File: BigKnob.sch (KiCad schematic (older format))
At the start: 10 parts, among them J1 NSJ12HF-1, J2 NSJ12HF-1, J3 NSJ12HF-1, J4 STEREO-JACK-SWITCHED-5-Pin, J5 STEREO-JACK-SWITCHED-5-Pin

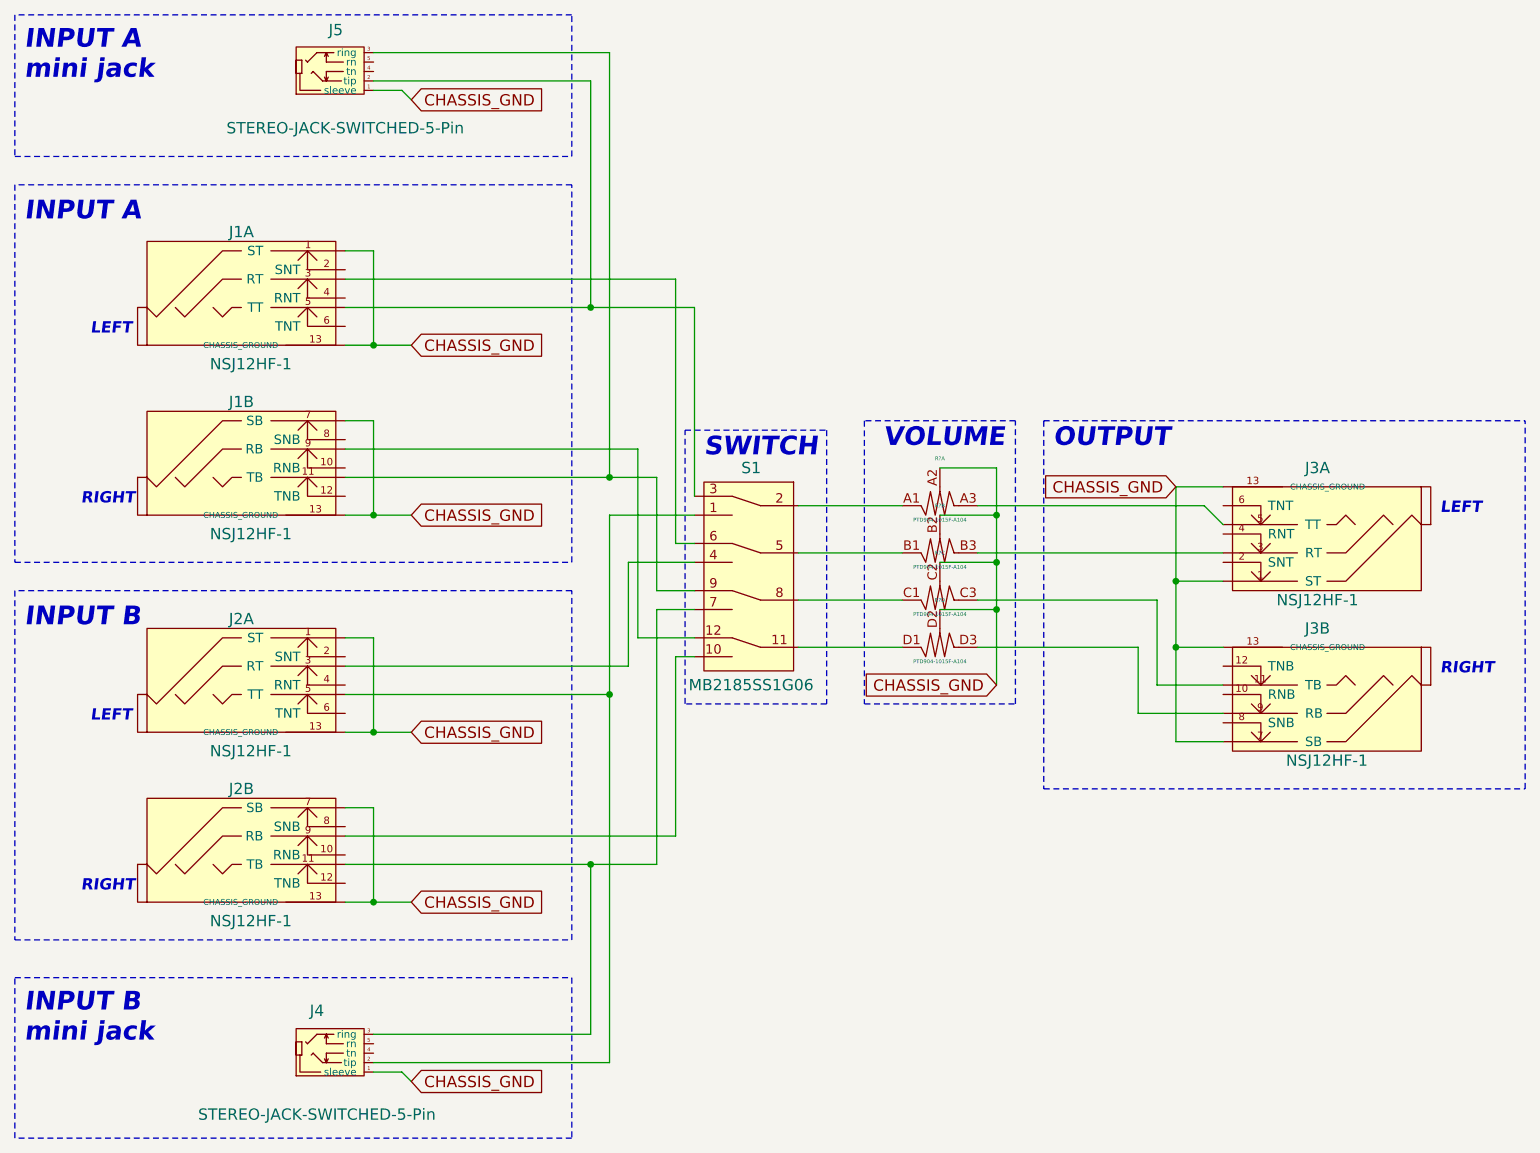
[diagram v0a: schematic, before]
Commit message: :punch: fixed schema
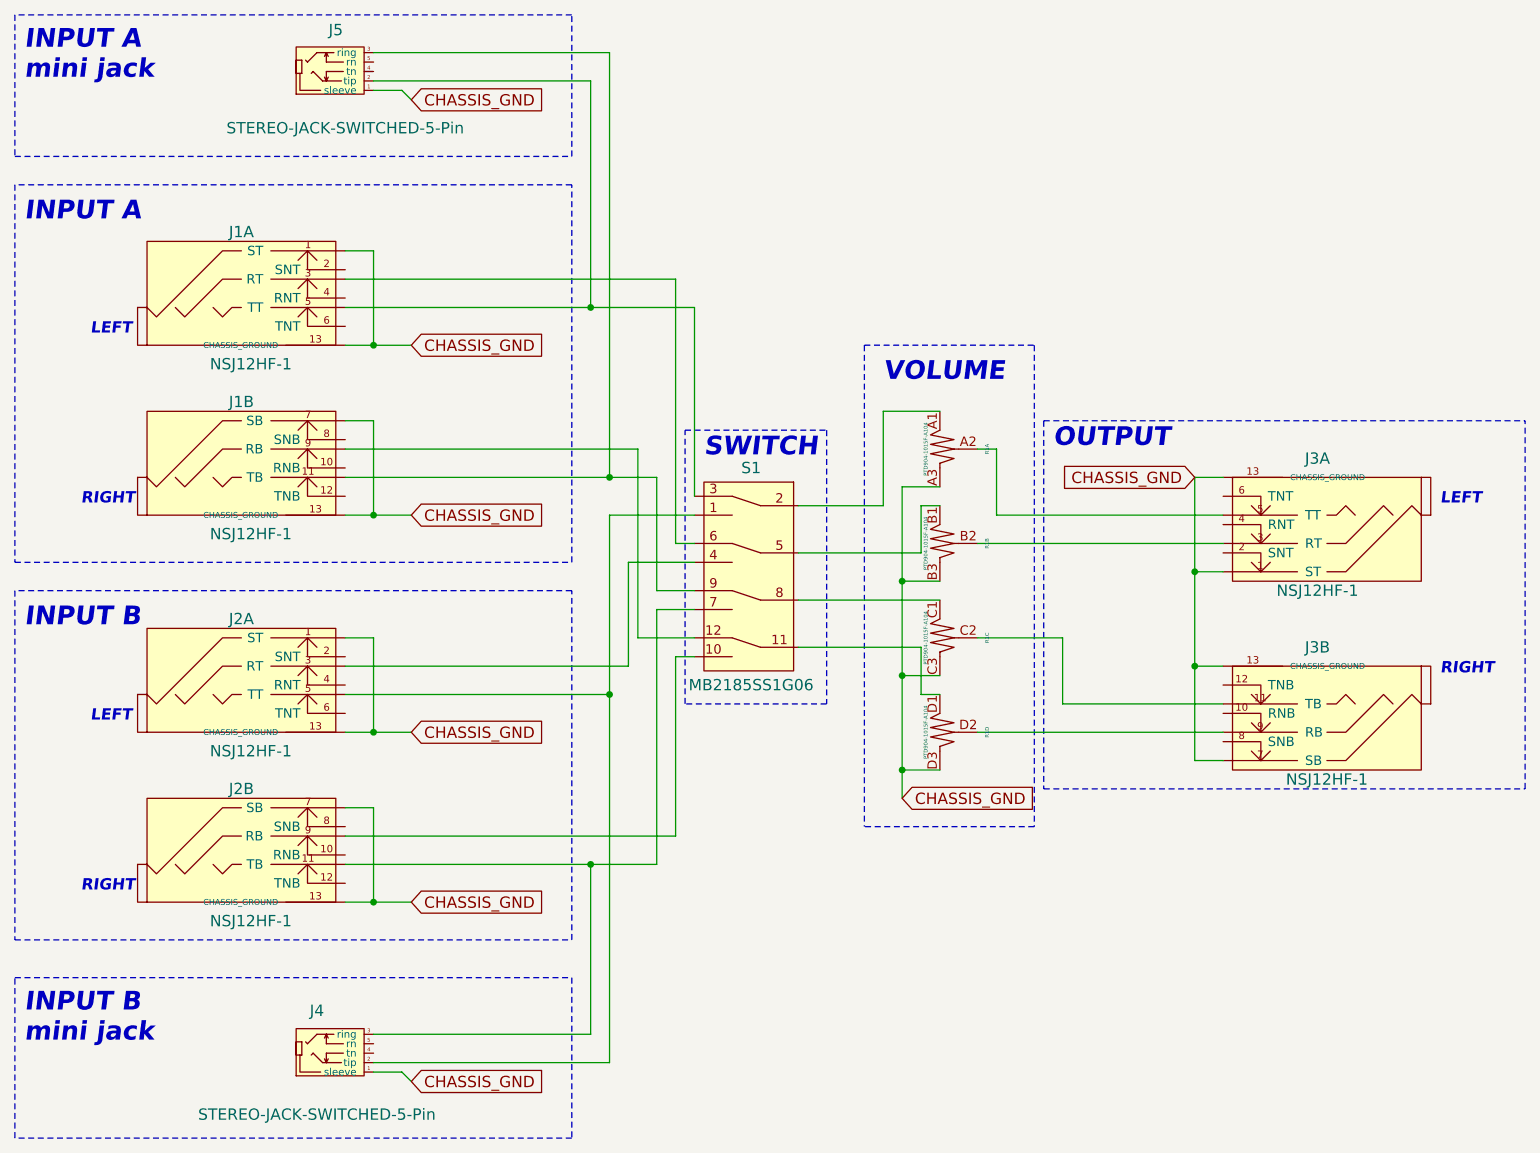
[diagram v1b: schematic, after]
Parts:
- R1: renamed from R?; footprint (none) -> stahllabs:PTD904-1015F-A104
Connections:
- net CHASSIS_GND: now also R1.A3, R1.B3, R1.C3, R1.D3; no longer R1.A2, R1.B2, R1.C2, R1.D2
- net at J3.3 (RT): now also R1.B2; no longer R1.B3
- net at J3.5 (TT): now also R1.A2; no longer R1.A3
- net at J3.11 (TB): now also R1.C2; no longer R1.C3
- net at J3.9 (RB): now also R1.D2; no longer R1.D3
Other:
- moved on the sheet: J3A, J3B, R1A, R1B, R1C, R1D
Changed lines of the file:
@@
 $EndComp
 Wire Wire Line
-	3150 2700 3300 2700
-Wire Wire Line
-	3300 2700 3500 2700
-Wire Wire Line
-	3150 3600 3300 3600
-Wire Wire Line
-	3300 3600 3500 3600
-Wire Wire Line
-	3150 4750 3300 4750
-Wire Wire Line
-	3300 4750 3500 4750
+	3150 2700 3500 2700
+Wire Wire Line
+	3150 3600 3500 3600
+Wire Wire Line
+	3150 4750 3500 4750
 Text GLabel 3500 2700 2    60   Input ~ 0
 CHASSIS_GND
@@
 CHASSIS_GND
 Wire Wire Line
-	3150 5650 3300 5650
-Wire Wire Line
-	3300 5650 3500 5650
+	3150 5650 3500 5650
 Text GLabel 3500 5650 2    60   Input ~ 0
 CHASSIS_GND
@@
 L NSJ12HF-1 J3
 U 1 1 58E15C9F
-P 8350 3750
-F 0 "J3" H 8400 3350 60  0000 C CNN
-F 1 "NSJ12HF-1" H 8400 4050 60  0000 C CNN
-F 2 "stahllabs:NSJ12HF-1" H 8700 3900 60  0001 C CNN
-F 3 "http://www.neutrik.com/en/audio/plugs-and-jacks/stacking-jacks/nsj12hf-1" H 8400 3250 21  0001 C BIN
-	1    8350 3750
+P 8350 3700
+F 0 "J3" H 8400 3300 60  0000 C CNN
+F 1 "NSJ12HF-1" H 8400 4000 60  0000 C CNN
+F 2 "stahllabs:NSJ12HF-1" H 8700 3850 60  0001 C CNN
+F 3 "http://www.neutrik.com/en/audio/plugs-and-jacks/stacking-jacks/nsj12hf-1" H 8400 3200 21  0001 C BIN
+	1    8350 3700
 	-1   0    0    1
 $EndComp
@@
 L NSJ12HF-1 J3
 U 2 1 58E15D3A
-P 8350 4600
-F 0 "J3" H 8400 4200 60  0000 C CNN
-F 1 "NSJ12HF-1" H 8350 4900 60  0000 C CNN
-F 2 "stahllabs:NSJ12HF-1" H 8700 4750 60  0001 C CNN
-F 3 "http://www.neutrik.com/en/audio/plugs-and-jacks/stacking-jacks/nsj12hf-1" H 8400 4100 21  0001 C BIN
-	2    8350 4600
+P 8350 4700
+F 0 "J3" H 8400 4300 60  0000 C CNN
+F 1 "NSJ12HF-1" H 8350 5000 60  0000 C CNN
+F 2 "stahllabs:NSJ12HF-1" H 8700 4850 60  0001 C CNN
+F 3 "http://www.neutrik.com/en/audio/plugs-and-jacks/stacking-jacks/nsj12hf-1" H 8400 4200 21  0001 C BIN
+	2    8350 4700
 	-1   0    0    1
 $EndComp
 Wire Wire Line
-	7450 4050 7450 4500
-Wire Wire Line
-	7450 4500 7800 4500
-Wire Wire Line
-	7350 4300 7350 4650
-Wire Wire Line
-	7350 4650 7800 4650
+	6950 4250 6950 4600
+Wire Wire Line
+	6950 4600 7800 4600
+Wire Wire Line
+	6500 4750 7800 4750
 Wire Wire Line
 	3150 4550 4550 4550
 Wire Wire Line
-	4550 3600 4550 4550
-Wire Wire Line
-	4550 4550 4550 6500
-Wire Wire Line
-	6500 3550 7700 3550
-Wire Wire Line
-	7700 3550 7800 3650
-Text Notes 8950 3600 0    60   Italic 12
+	4550 3600 4550 6500
+Text Notes 8950 3550 0    60   Italic 12
 LEFT
 Text Notes 1800 2650 0    60   Italic 12
@@
 RIGHT
 Wire Wire Line
-	6500 3800 7800 3800
-Wire Wire Line
-	7550 4300 7800 4300
-Wire Wire Line
-	7550 3450 7550 3950
-Wire Wire Line
-	7550 3950 7550 4300
-Wire Wire Line
-	7550 4300 7550 4800
-Wire Wire Line
-	7800 3950 7550 3950
-Connection ~ 7550 3950
-Wire Wire Line
-	7550 4800 7800 4800
-Connection ~ 7550 4300
-Wire Wire Line
-	6500 4050 7450 4050
-Wire Wire Line
-	6500 4300 7350 4300
+	7650 4400 7800 4400
+Wire Wire Line
+	7650 3400 7650 4900
+Wire Wire Line
+	7800 3900 7650 3900
+Connection ~ 7650 3900
+Wire Wire Line
+	7650 4900 7800 4900
+Connection ~ 7650 4400
 Text Notes 8950 4450 0    60   Italic 12
 RIGHT
 Wire Wire Line
-	3150 2500 4450 2500
-Wire Wire Line
-	4450 2500 5000 2500
+	3150 2500 5000 2500
 Wire Wire Line
 	5000 2500 5000 3500
@@
 Connection ~ 3300 3600
 Wire Wire Line
-	7550 3450 7800 3450
-Text GLabel 7550 3450 0    60   Input ~ 0
-CHASSIS_GND
-Wire Wire Line
-	3150 3400 4550 3400
-Wire Wire Line
-	4550 3400 4800 3400
+	7650 3400 7800 3400
+Text GLabel 7650 3400 0    60   Input ~ 0
+CHASSIS_GND
+Wire Wire Line
+	3150 3400 4800 3400
 Wire Wire Line
 	4800 3400 4800 4000
@@
 	4800 4000 5000 4000
 Wire Wire Line
-	3150 5450 4450 5450
-Wire Wire Line
-	4450 5450 4800 5450
+	3150 5450 4800 5450
 Wire Wire Line
 	4800 5450 4800 4100
@@
 INPUT A\nmini jack
 Wire Wire Line
-	5550 3550 6100 3550
-Wire Wire Line
-	5550 3800 6100 3800
-Wire Wire Line
-	5550 4050 6100 4050
-Wire Wire Line
-	5550 4300 6100 4300
-Wire Wire Line
-	6300 3350 6600 3350
-Wire Wire Line
-	6600 3350 6600 3600
-Wire Wire Line
-	6600 3600 6600 3850
-Wire Wire Line
-	6600 3850 6600 4100
-Wire Wire Line
-	6600 4100 6600 4500
-Text GLabel 6600 4500 0    60   Input ~ 0
-CHASSIS_GND
-Wire Wire Line
-	6300 3600 6600 3600
-Connection ~ 6600 3600
-Wire Wire Line
-	6300 3850 6600 3850
-Wire Wire Line
-	6600 3850 6600 3850
-Connection ~ 6600 3850
-Wire Wire Line
-	6300 4100 6600 4100
-Connection ~ 6600 4100
-$Comp
-L PTD904-1015F-A104 R?
+	5550 4050 6300 4050
+Text GLabel 6100 5100 2    60   Input ~ 0
+CHASSIS_GND
+$Comp
+L PTD904-1015F-A104 R1
 U 1 1 58FEAB86
-P 6300 3550
-F 0 "R?" H 6300 3800 20  0000 C CNN
-F 1 "PTD904-1015F-A104" H 6300 3475 20  0000 C CNN
-F 2 "" H 6300 3550 60  0001 C CNN
-F 3 "" H 6300 3550 60  0001 C CNN
-	1    6300 3550
-	1    0    0    -1
-$EndComp
-$Comp
-L PTD904-1015F-A104 R?
+P 6300 3250
+F 0 "R1" H 6300 3500 20  0000 C CNN
+F 1 "PTD904-1015F-A104" H 6300 3175 20  0000 C CNN
+F 2 "stahllabs:PTD904-1015F-A104" H 6300 3250 60  0001 C CNN
+F 3 "" H 6300 3250 60  0001 C CNN
+	1    6300 3250
+	0    1    1    0
+$EndComp
+$Comp
+L PTD904-1015F-A104 R1
 U 2 1 58FEABBF
-P 6300 3800
-F 0 "R?" H 6300 4050 20  0000 C CNN
-F 1 "PTD904-1015F-A104" H 6300 3725 20  0000 C CNN
-F 2 "" H 6300 3800 60  0001 C CNN
-F 3 "" H 6300 3800 60  0001 C CNN
-	2    6300 3800
-	1    0    0    -1
-$EndComp
-$Comp
-L PTD904-1015F-A104 R?
-U 3 1 58FEAC45
-P 6300 4050
-F 0 "R?" H 6300 4300 20  0000 C CNN
-F 1 "PTD904-1015F-A104" H 6300 3975 20  0000 C CNN
-F 2 "" H 6300 4050 60  0001 C CNN
-F 3 "" H 6300 4050 60  0001 C CNN
-	3    6300 4050
-	1    0    0    -1
-$EndComp
-$Comp
-L PTD904-1015F-A104 R?
+P 6300 3750
+F 0 "R1" H 6300 4000 20  0000 C CNN
+F 1 "PTD904-1015F-A104" H 6300 3675 20  0000 C CNN
+F 2 "stahllabs:PTD904-1015F-A104" H 6300 3750 60  0001 C CNN
+F 3 "" H 6300 3750 60  0001 C CNN
+	2    6300 3750
+	0    1    1    0
+$EndComp
+$Comp
+L PTD904-1015F-A104 R1
 U 4 1 58FEAC80
-P 6300 4300
-F 0 "R?" H 6300 4550 20  0000 C CNN
-F 1 "PTD904-1015F-A104" H 6300 4225 20  0000 C CNN
-F 2 "" H 6300 4300 60  0001 C CNN
-F 3 "" H 6300 4300 60  0001 C CNN
-	4    6300 4300
-	1    0    0    -1
+P 6300 4750
+F 0 "R1" H 6300 5000 20  0000 C CNN
+F 1 "PTD904-1015F-A104" H 6300 4675 20  0000 C CNN
+F 2 "stahllabs:PTD904-1015F-A104" H 6300 4750 60  0001 C CNN
+F 3 "" H 6300 4750 60  0001 C CNN
+	4    6300 4750
+	0    1    1    0
 $EndComp
 Wire Notes Line
@@
 SWITCH
 Wire Notes Line
-	5900 4600 6700 4600
-Wire Notes Line
-	6700 4600 6700 3100
-Wire Notes Line
-	6700 3100 5900 3100
-Wire Notes Line
-	5900 3100 5900 4600
-Text Notes 6000 3250 0    99   Italic 20
+	5900 2700 6800 2700
+Wire Notes Line
+	5900 2700 5900 5250
+Text Notes 6000 2900 0    99   Italic 20
 VOLUME
+Wire Wire Line
+	6600 3250 6600 3600
+Wire Wire Line
+	6600 3600 7800 3600
+Wire Wire Line
+	6500 3750 7800 3750
+$Comp
+L PTD904-1015F-A104 R1
+U 3 1 58FEAC45
+P 6300 4250
+F 0 "R1" H 6300 4500 20  0000 C CNN
+F 1 "PTD904-1015F-A104" H 6300 4175 20  0000 C CNN
+F 2 "stahllabs:PTD904-1015F-A104" H 6300 4250 60  0001 C CNN
+F 3 "" H 6300 4250 60  0001 C CNN
+	3    6300 4250
+	0    1    1    0
+$EndComp
+Wire Wire Line
+	5550 3550 6000 3550
+Wire Wire Line
+	6000 3550 6000 3050
+Wire Wire Line
+	6000 3050 6300 3050
+Wire Wire Line
+	6500 3250 6600 3250
+Wire Wire Line
+	5550 4300 6200 4300
+Wire Wire Line
+	6200 4300 6200 4550
+Wire Wire Line
+	6200 4550 6300 4550
+Wire Wire Line
+	5550 3800 6200 3800
+Wire Wire Line
+	6200 3800 6200 3550
+Wire Wire Line
+	6200 3550 6300 3550
+Wire Notes Line
+	6800 2700 6800 5250
+Wire Wire Line
+	7450 3750 7450 3750
+Wire Wire Line
+	6950 4250 6500 4250
+Wire Wire Line
+	6100 3450 6100 5100
+Wire Wire Line
+	6100 3450 6300 3450
+Wire Wire Line
+	6300 3950 6100 3950
+Connection ~ 6100 3950
+Wire Wire Line
+	6300 4450 6100 4450
+Connection ~ 6100 4450
+Wire Wire Line
+	6300 4950 6100 4950
+Connection ~ 6100 4950
+Wire Notes Line
+	6800 5250 5900 5250
 $EndSCHEMATC
